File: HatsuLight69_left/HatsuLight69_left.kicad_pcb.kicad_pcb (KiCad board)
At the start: 2 copper layers, 164.5 x 124 mm, 133 parts, among them J1 USB_C_Receptacle, J2 MJ-4PP-9, J3 I2C, J4 SPI, SW1 SW_PUSH, SW10 SW_PUSH-kbd, SW11 SW_PUSH-kbd, SW12 SW_PUSH-kbd, SW13 SW_PUSH-kbd, SW14 SW_PUSH-kbd, SW15 SW_PUSH-kbd, SW16 SW_PUSH-kbd, SW17 SW_PUSH-kbd, SW18 SW_PUSH-kbd, SW19 SW_PUSH-kbd, SW2 SW_PUSH-kbd, SW20 SW_PUSH-kbd, SW21 SW_PUSH-kbd, SW22 SW_PUSH-kbd, SW23 SW_PUSH-kbd, SW24 SW_PUSH-kbd, SW25 SW_PUSH-kbd, SW26 SW_PUSH-kbd, SW27 SW_PUSH-kbd, SW28 SW_PUSH-kbd, SW29 SW_PUSH-kbd, SW3 SW_PUSH-kbd, SW30 SW_PUSH-kbd, SW31 SW_PUSH-kbd, SW32 SW_PUSH-kbd, SW33 SW_PUSH-kbd, SW4 SW_PUSH-kbd, SW5 SW_PUSH-kbd, SW6 SW_PUSH-kbd, SW7 SW_PUSH-kbd, SW8 SW_PUSH-kbd, SW9 SW_PUSH-kbd, U1 ATMEGA32U4, X1 CSTNE16M0V530000R0

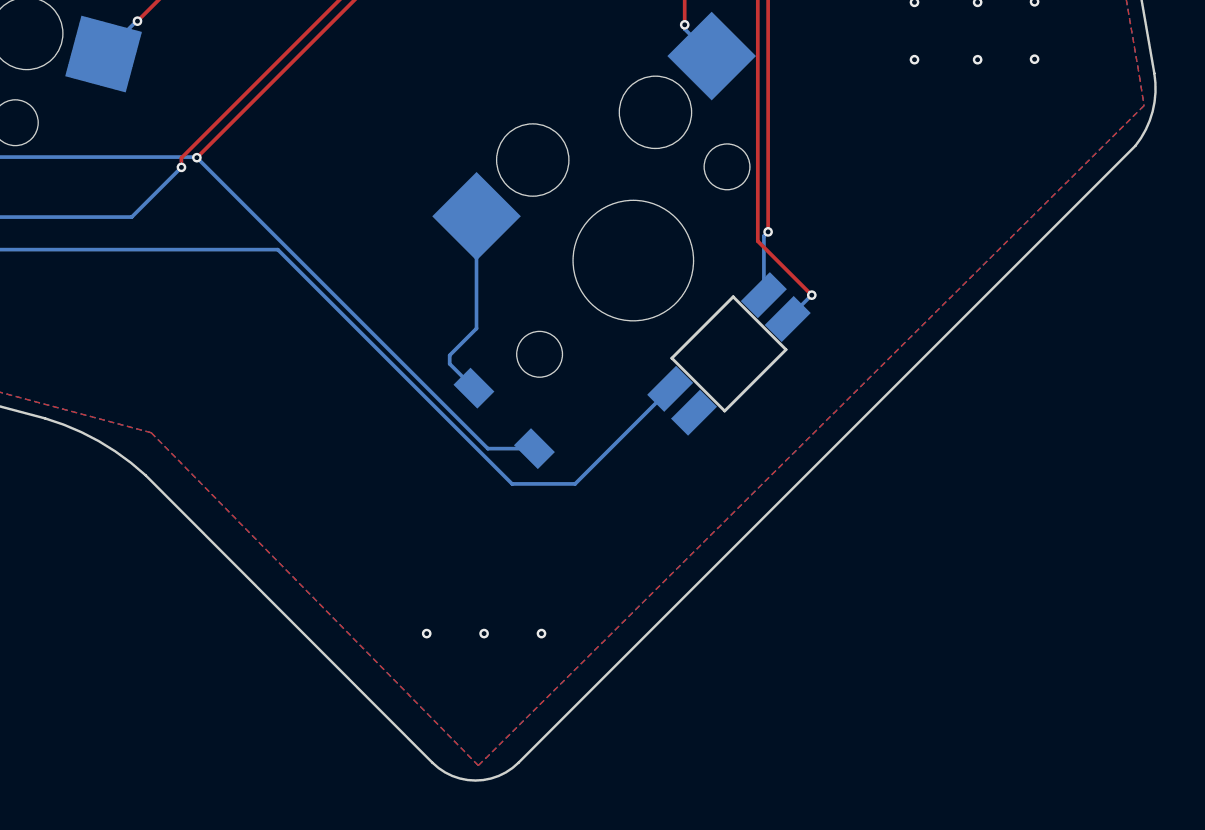
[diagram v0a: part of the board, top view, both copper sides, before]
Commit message: update
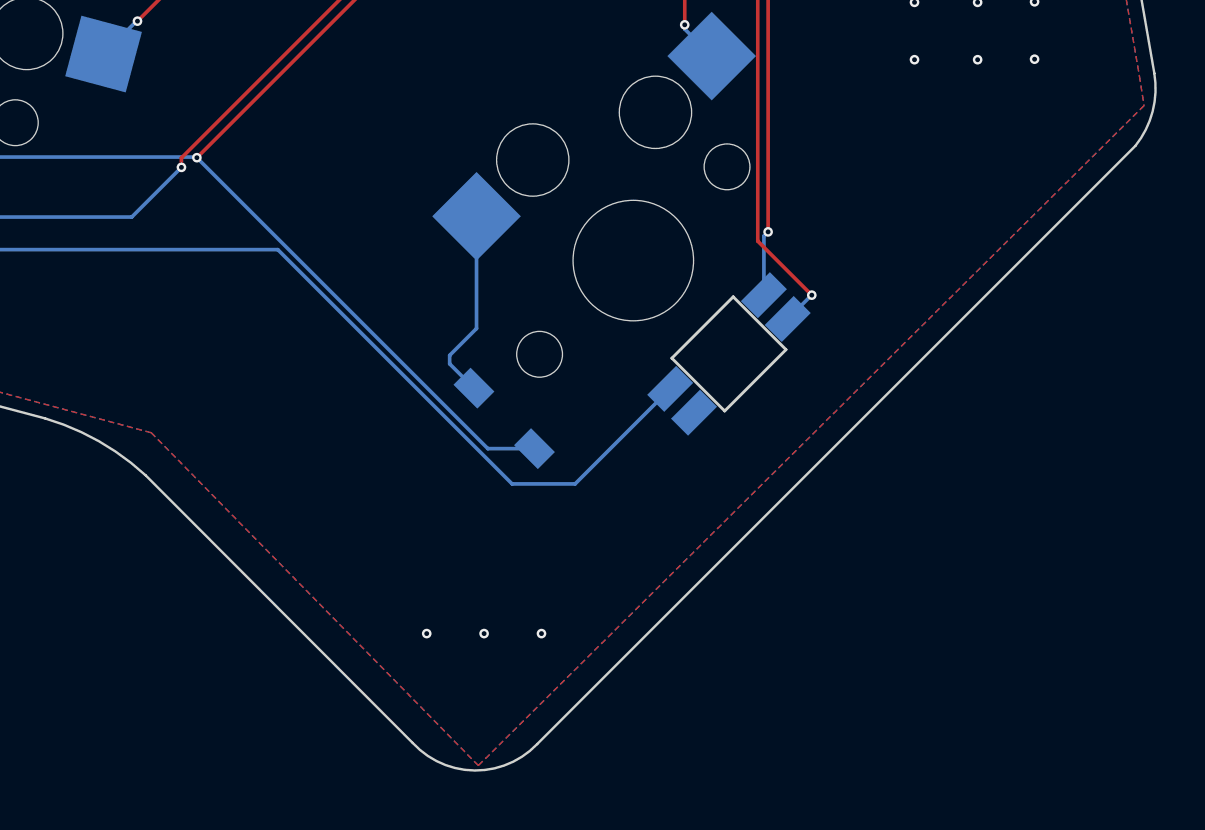
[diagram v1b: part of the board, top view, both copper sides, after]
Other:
- board size 164.5 x 124 mm -> 164.5 x 123.6 mm
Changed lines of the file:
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@@
   (gr_line (start 47.62514 35.71886) (end 47.62514 125.01581) (layer "Edge.Cuts") (width 0.1))
   (gr_arc (start 212.119649 124.389144) (mid 212.048446 125.976583) (end 211.336215 127.397062) (layer "Edge.Cuts") (width 0.1))
-  (gr_line (start 170.27102 141.076908) (end 182.165878 152.995521) (layer "Edge.Cuts") (width 0.1))
   (gr_arc (start 133.945525 130.96894) (mid 136.350312 131.090679) (end 138.730511 131.454651) (layer "Edge.Cuts") (width 0.1))
-  (gr_line (start 185.737756 152.995521) (end 211.336215 127.397062) (layer "Edge.Cuts") (width 0.1))
   (gr_arc (start 191.690886 29.76573) (mid 194.842723 30.957889) (end 196.416613 33.937518) (layer "Edge.Cuts") (width 0.1))
+  (gr_line (start 170.27102 141.076908) (end 181.349466 152.177417) (layer "Edge.Cuts") (width 0.1))
   (gr_line (start 191.542443 29.765732) (end 191.003069 29.765732) (layer "Edge.Cuts") (width 0.1))
   (gr_arc (start 166.092427 138.708009) (mid 168.318349 139.651459) (end 170.27102 141.076908) (layer "Edge.Cuts") (width 0.1))
+  (gr_arc (start 186.512199 152.222199) (mid 183.92113 153.318406) (end 181.349466 152.177417) (layer "Edge.Cuts") (width 0.1))
   (gr_arc (start 53.57827 130.96894) (mid 49.368771 129.225309) (end 47.62514 125.01581) (layer "Edge.Cuts") (width 0.1))
-  (gr_arc (start 185.737756 152.995521) (mid 183.951817 153.735281) (end 182.165878 152.995521) (layer "Edge.Cuts") (width 0.1))
   (gr_line (start 179.933069 29.765732) (end 53.57827 29.76573) (layer "Edge.Cuts") (width 0.1))
   (gr_line (start 130.96896 130.96894) (end 133.945525 130.96894) (layer "Edge.Cuts") (width 0.1))
   (gr_line (start 191.542443 29.765732) (end 191.690886 29.76573) (layer "Edge.Cuts") (width 0.1))
+  (gr_line (start 186.512199 152.222199) (end 211.336215 127.397062) (layer "Edge.Cuts") (width 0.1))
   (gr_line (start 53.57827 130.96894) (end 130.96896 130.96894) (layer "Edge.Cuts") (width 0.1))
   (gr_arc (start 47.62514 35.71886) (mid 49.368771 31.509361) (end 53.57827 29.76573) (layer "Edge.Cuts") (width 0.1))

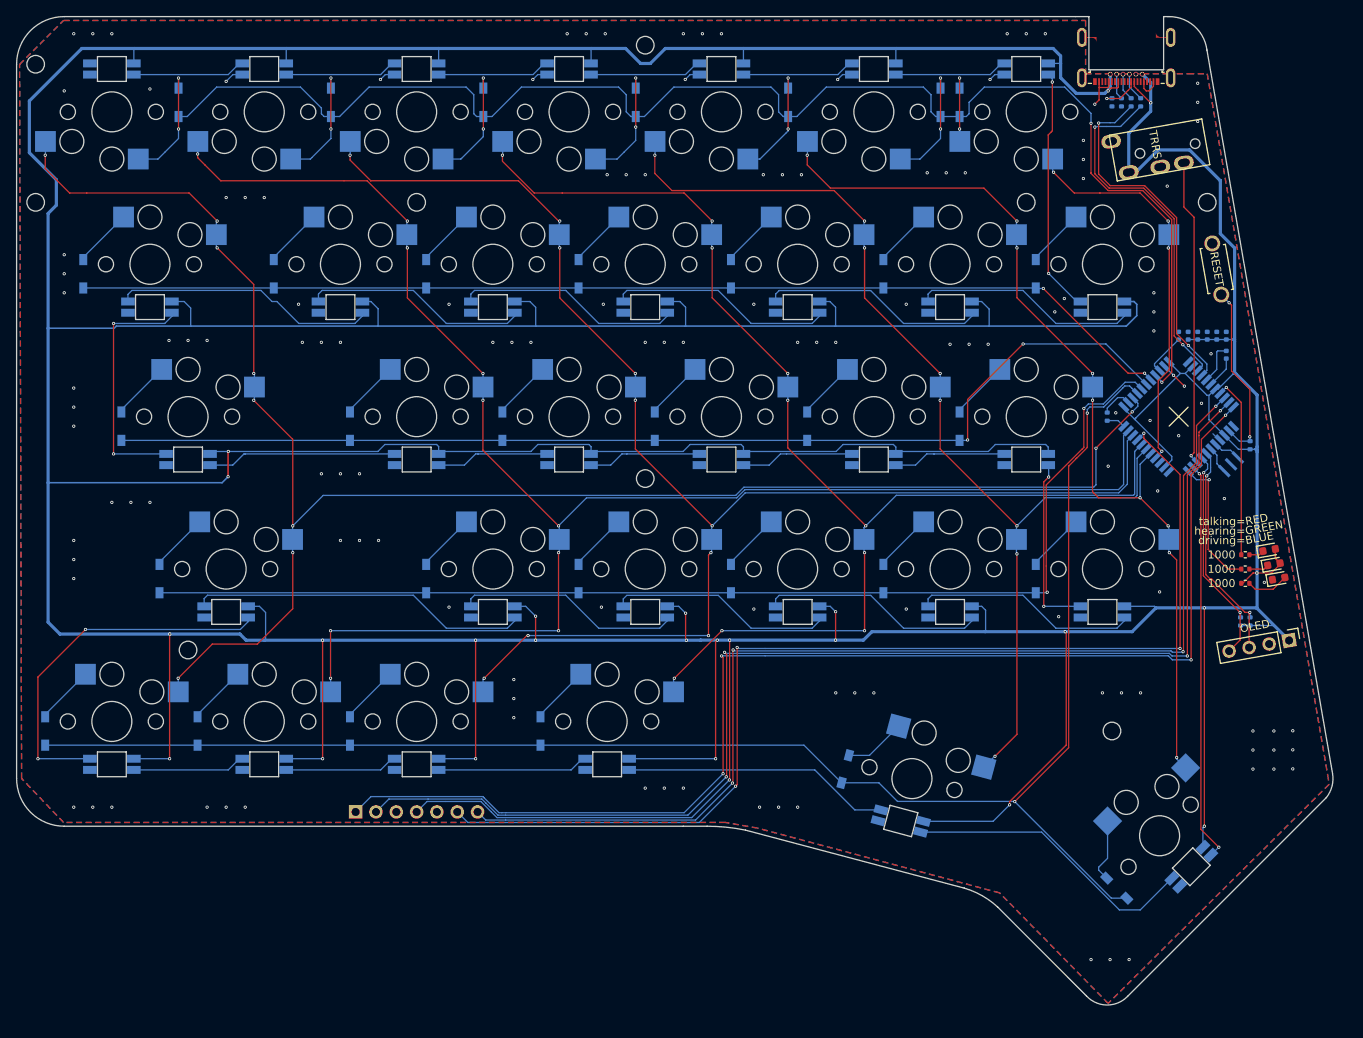
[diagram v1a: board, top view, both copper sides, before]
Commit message: update
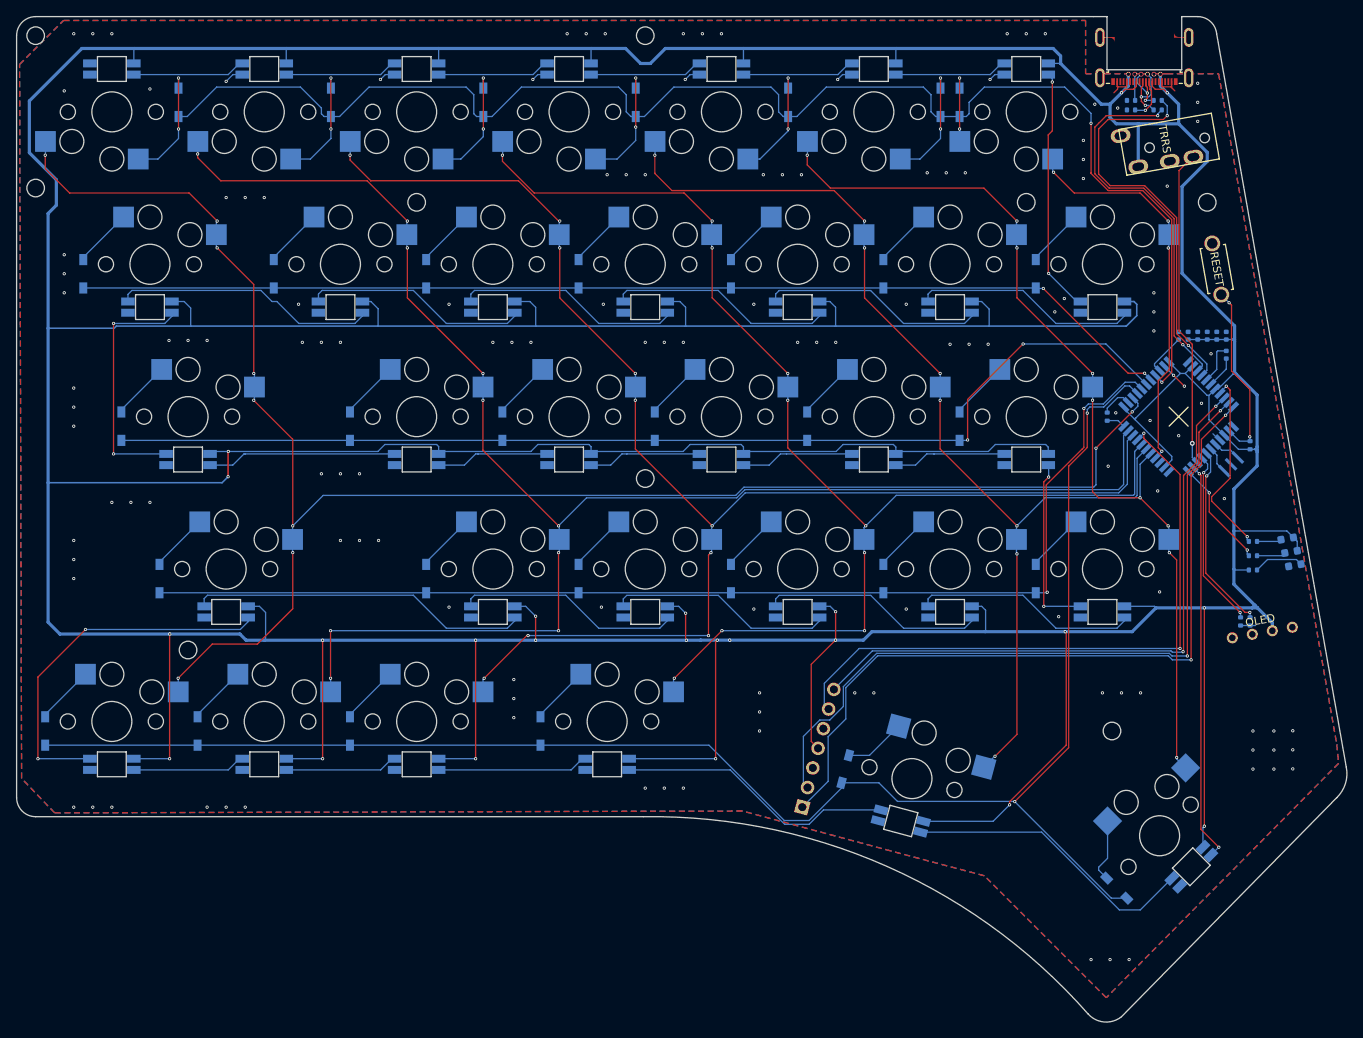
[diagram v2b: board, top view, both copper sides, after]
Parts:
- D1, D2, D3, R5, R8, R9: moved to B.Cu
- J3: footprint Connector_PinHeader_2.54mm:PinHeader_1x04_P2.54mm_Vertical -> kbd:OLED_v2
- moved J4 55.8 mm to (145.8, 128.6), turned to -15 degrees
- moved ? 3.57 mm to (50.0, 32.1)
- moved J3 3.50 mm to (203.3, 106.8), turned to 10 degrees
- moved R4 3.33 mm to (190.3, 40.2), turned to 0 degrees
- moved D1 2.68 mm to (206.5, 95.0)
- moved D2 2.64 mm to (206.9, 96.7)
- moved D3 2.62 mm to (207.4, 98.3)
- moved R1 2.57 mm to (186.9, 41.4), turned to 180 degrees
- moved R3 2.33 mm to (190.3, 41.4), turned to 0 degrees
- moved J1 2.26 mm to (188.6, 32.1)
- moved R8 1.92 mm to (202.2, 97.2)
- moved R9 1.92 mm to (202.2, 98.9)
- moved R5 1.92 mm to (202.2, 95.4)
- moved ? 1.79 mm to (50.0, 51.2)
- moved J2 1.39 mm to (197.6, 44.7)
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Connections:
- J1 pad A6: (no net) -> Net-(J1-PadA6)
- J1 pad A7: (no net) -> Net-(J1-PadA7)
- J3 pad 1: VCC -> SDA
- J3 pad 2: GND -> SCL
- J3 pad 3: SCL -> VCC
- J3 pad 4: SDA -> GND
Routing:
- net SCLK: track 141.2 -> 79.6 mm, vias 4 -> 2
- net MISO: track 157.1 -> 96.0 mm, vias 4 -> 2
- net MOSI: track 154.9 -> 94.4 mm, vias 4 -> 2
- net NCS: track 140.0 -> 79.7 mm, vias 4 -> 2
- net VCC: track 1088.7 -> 1052.4 mm, vias 25 -> 23
- net /MCU/D+: track 44.9 -> 50.6 mm
- net SDA: track 27.8 -> 22.4 mm
- net Net-(J1-PadA7): track 3.59 -> 8.58 mm, vias 0 -> 2
- net SCL: track 28.1 -> 23.6 mm
- net ROW4: track 203.8 -> 208.0 mm
- net Net-(R8-Pad2): track 17.0 -> 13.7 mm, vias 1 -> 2
- net Net-(J1-PadA6): track 3.42 -> 6.66 mm, vias 0 -> 2
- net /MCU/D-: track 45.6 -> 48.2 mm
- net ROW0: track 182.3 -> 180.6 mm
- net Net-(D37-Pad1): track 33.5 -> 35.0 mm
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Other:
- board size 164.5 x 123.6 mm -> 166.3 x 125.7 mm
- board text added: "=driving"
- board text added: "=hearing"
- board text added: "=talking"
- board text removed: "OLED"
- board text removed: "driving="
- board text removed: "hearing="
- board text removed: "talking="
